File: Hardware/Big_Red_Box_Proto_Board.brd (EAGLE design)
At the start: 0.3 x 65.9 mm, 5 parts

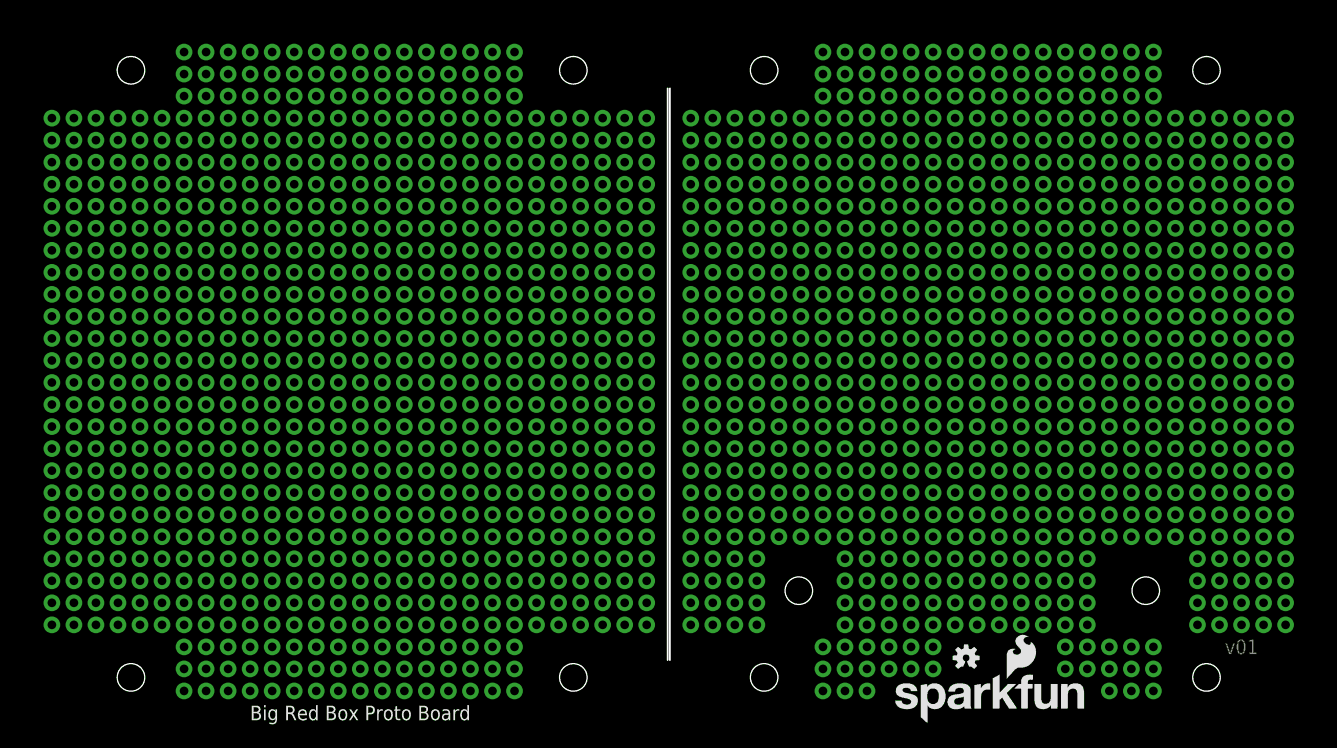
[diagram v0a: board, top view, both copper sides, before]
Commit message: board cleanup
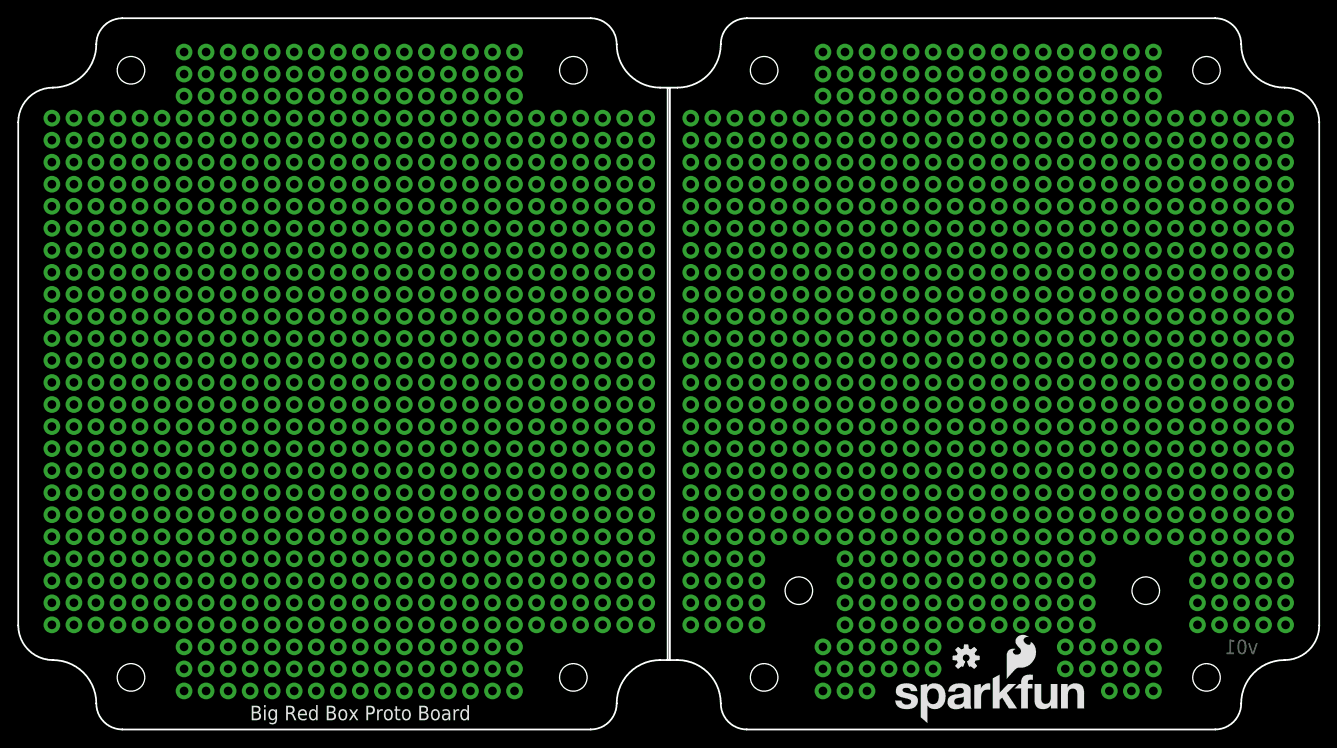
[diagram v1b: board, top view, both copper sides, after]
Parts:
- E$1: device SparkFun-Boards:FLANGED_RED_ENCLOSURE-OUTLINE -> SparkFun-Boards:FLANGED_RED_ENCLOSURE-DIMENSION
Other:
- board size 0.3 x 65.9 mm -> 150 x 82 mm
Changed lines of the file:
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@@
 <text x="-35.56" y="-38.1" size="1.6764" layer="21" font="vector" ratio="15" align="center">Big Red Box Proto Board</text>
 <text x="-35.56" y="-38.1" size="1.6764" layer="22" font="vector" ratio="15" rot="MR0" align="center">Big Red Box Proto Board</text>
-<text x="66.04" y="-30.48" size="1.6764" layer="1" font="vector" ratio="15" align="center">v01</text>
+<text x="66.04" y="-30.48" size="1.6764" layer="16" font="vector" ratio="15" rot="MR0" align="center">v01</text>
 <wire x1="0.127" y1="33.909" x2="0.127" y2="-32.004" width="0.2032" layer="20"/>
 <wire x1="-0.127" y1="33.909" x2="-0.127" y2="-32.004" width="0.2032" layer="20"/>
@@
 </autorouter>
 <elements>
-<element name="E$1" library="SparkFun-Boards" package="FLANGED_RED_ENCLOSURE-OUTLINE" value="" x="-75" y="-40"/>
+<element name="E$1" library="SparkFun-Boards" package="FLANGED_RED_ENCLOSURE-DIMENSION" value="" x="-75" y="-40"/>
 <element name="E$2" library="SparkFun-Aesthetics" package="SFE_LOGO_NAME_FLAME_.2" value="" x="25.4" y="-39.37"/>
 <element name="E$3" library="SparkFun-Aesthetics" package="SFE_LOGO_NAME_FLAME_.2" value="" x="49.53" y="-39.37" rot="MR0"/>
@@
 <via x="53.34" y="30.48" extent="1-16" drill="1" diameter="1.9304"/>
 </signal>
-<signal name="S$281">
-<wire x1="0" y1="27.94" x2="0" y2="27.94" width="0" layer="19" extent="1-16"/>
-</signal>
-<signal name="S$282">
-<wire x1="0" y1="25.4" x2="0" y2="25.4" width="0" layer="19" extent="1-16"/>
-</signal>
-<signal name="S$283">
-<wire x1="0" y1="22.86" x2="0" y2="22.86" width="0" layer="19" extent="1-16"/>
-</signal>
-<signal name="S$284">
-<wire x1="0" y1="20.32" x2="0" y2="20.32" width="0" layer="19" extent="1-16"/>
-</signal>
-<signal name="S$285">
-<wire x1="0" y1="17.78" x2="0" y2="17.78" width="0" layer="19" extent="1-16"/>
-</signal>
-<signal name="S$286">
-<wire x1="0" y1="15.24" x2="0" y2="15.24" width="0" layer="19" extent="1-16"/>
-</signal>
-<signal name="S$287">
-<wire x1="0" y1="12.7" x2="0" y2="12.7" width="0" layer="19" extent="1-16"/>
-</signal>
-<signal name="S$288">
-<wire x1="0" y1="10.16" x2="0" y2="10.16" width="0" layer="19" extent="1-16"/>
-</signal>
-<signal name="S$289">
-<wire x1="0" y1="-12.7" x2="0" y2="-12.7" width="0" layer="19" extent="1-16"/>
-</signal>
-<signal name="S$290">
-<wire x1="0" y1="-7.62" x2="0" y2="-7.62" width="0" layer="19" extent="1-16"/>
-</signal>
-<signal name="S$416">
-<wire x1="0" y1="-2.54" x2="0" y2="-2.54" width="0" layer="19" extent="1-16"/>
-</signal>
-<signal name="S$419">
-<wire x1="0" y1="2.54" x2="0" y2="2.54" width="0" layer="19" extent="1-16"/>
-</signal>
-<signal name="S$420">
-<wire x1="0" y1="5.08" x2="0" y2="5.08" width="0" layer="19" extent="1-16"/>
-</signal>
-<signal name="S$422">
-<wire x1="0" y1="7.62" x2="0" y2="7.62" width="0" layer="19" extent="1-16"/>
-</signal>
-<signal name="S$423">
-<wire x1="0" y1="0" x2="0" y2="0" width="0" layer="19" extent="1-16"/>
-</signal>
-<signal name="S$424">
-<wire x1="0" y1="-27.94" x2="0" y2="-27.94" width="0" layer="19" extent="1-16"/>
-</signal>
-<signal name="S$425">
-<wire x1="0" y1="-25.4" x2="0" y2="-25.4" width="0" layer="19" extent="1-16"/>
-</signal>
-<signal name="S$426">
-<wire x1="0" y1="-22.86" x2="0" y2="-22.86" width="0" layer="19" extent="1-16"/>
-</signal>
-<signal name="S$430">
-<wire x1="0" y1="-20.32" x2="0" y2="-20.32" width="0" layer="19" extent="1-16"/>
-</signal>
-<signal name="S$445">
-<wire x1="0" y1="-17.78" x2="0" y2="-17.78" width="0" layer="19" extent="1-16"/>
-</signal>
-<signal name="S$651">
-<wire x1="0" y1="-15.24" x2="0" y2="-15.24" width="0" layer="19" extent="1-16"/>
-</signal>
-<signal name="S$940">
-<wire x1="0" y1="-10.16" x2="0" y2="-10.16" width="0" layer="19" extent="1-16"/>
-</signal>
-<signal name="S$941">
-<wire x1="0" y1="-5.08" x2="0" y2="-5.08" width="0" layer="19" extent="1-16"/>
-</signal>
 <signal name="S$193">
 <via x="10.16" y="-20.32" extent="1-16" drill="1" diameter="1.9304"/>
@@
 <via x="-2.54" y="30.48" extent="1-16" drill="1" diameter="1.9304"/>
 </signal>
-<signal name="S$1501">
-<wire x1="0" y1="30.48" x2="0" y2="30.48" width="0" layer="19" extent="1-16"/>
-</signal>
 <signal name="S$1502">

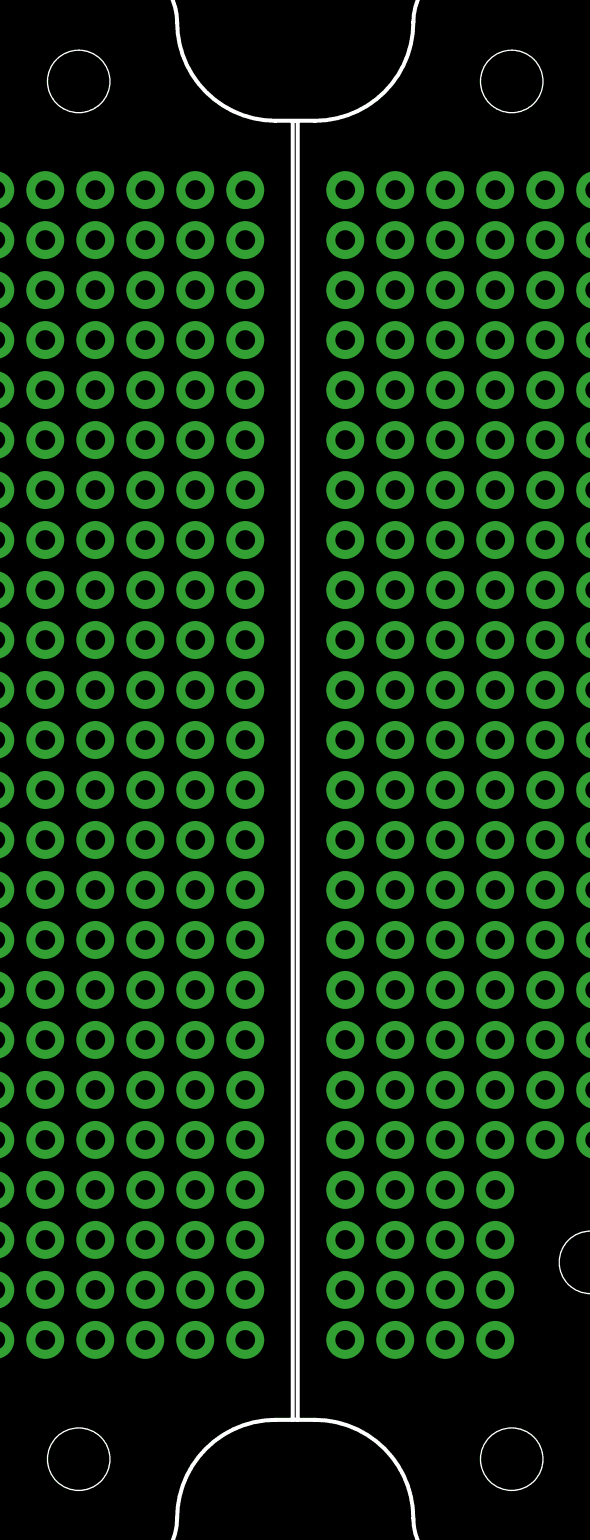
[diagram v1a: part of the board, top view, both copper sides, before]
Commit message: fixed vscore
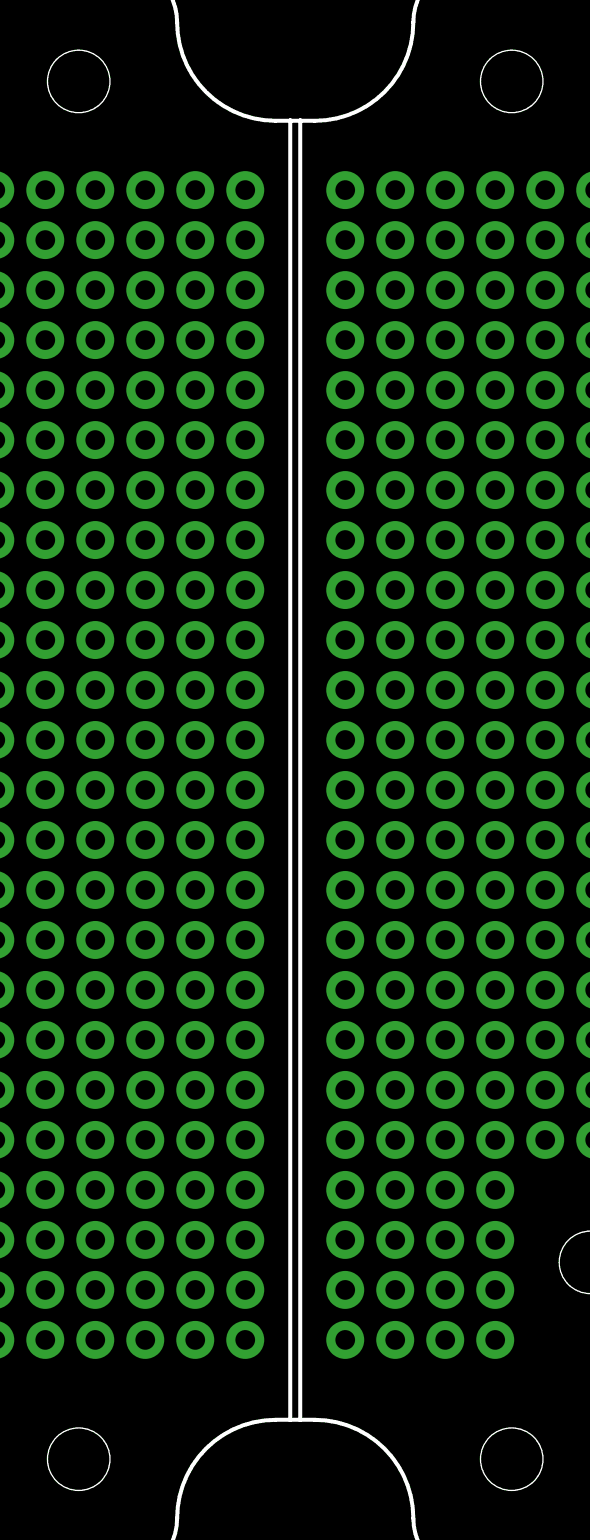
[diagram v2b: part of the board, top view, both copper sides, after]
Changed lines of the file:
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@@
 <?xml version="1.0" encoding="utf-8"?>
 <!DOCTYPE eagle SYSTEM "eagle.dtd">
-<eagle version="7.1.0">
+<eagle version="6.5.0">
 <drawing>
 <settings>
@@
 <setting verticaltext="up"/>
 </settings>
-<grid distance="0.005" unitdist="inch" unit="inch" style="lines" multiple="1" display="yes" altdistance="0.025" altunitdist="inch" altunit="inch"/>
+<grid distance="0.01" unitdist="inch" unit="inch" style="lines" multiple="1" display="yes" altdistance="0.025" altunitdist="inch" altunit="inch"/>
 <layers>
 <layer number="1" name="Top" color="4" fill="1" visible="yes" active="yes"/>
@@
 <text x="-35.56" y="-38.1" size="1.6764" layer="22" font="vector" ratio="15" rot="MR0" align="center">Big Red Box Proto Board</text>
 <text x="66.04" y="-30.48" size="1.6764" layer="16" font="vector" ratio="15" rot="MR0" align="center">v01</text>
-<wire x1="0.127" y1="33.909" x2="0.127" y2="-32.004" width="0.2032" layer="20"/>
-<wire x1="-0.127" y1="33.909" x2="-0.127" y2="-32.004" width="0.2032" layer="20"/>
+<wire x1="0.254" y1="34.036" x2="0.254" y2="-32.004" width="0.2032" layer="20"/>
+<wire x1="-0.254" y1="34.036" x2="-0.254" y2="-32.004" width="0.2032" layer="20"/>
 </plain>
 <attributes>
@@
 <pass name="Default">
 <param name="RoutingGrid" value="50mil"/>
-<param name="AutoGrid" value="1"/>
-<param name="Efforts" value="0"/>
-<param name="TopRouterVariant" value="1"/>
 <param name="tpViaShape" value="round"/>
 <param name="PrefDir.1" value="|"/>
